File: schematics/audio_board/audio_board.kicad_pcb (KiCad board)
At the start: 2 copper layers, 69 parts, among them J1 servo ctrl, J10 charge en, J3 power, J4 pyr ctrl, J5 servo out, J6 pyr in, J7 audio ctrl, J8 speaker, J9 battery, Q1 bc847, Q2 bc847, Q3 bc847, Q7 dgm2305ux, Q8 dgm2305ux, Q9 dgm2305ux, U1 TPS613222ADBV, U2 MAX98357A, U3 TPS613222ADBV, U4 TPS613222ADBV, U8 MCP73812

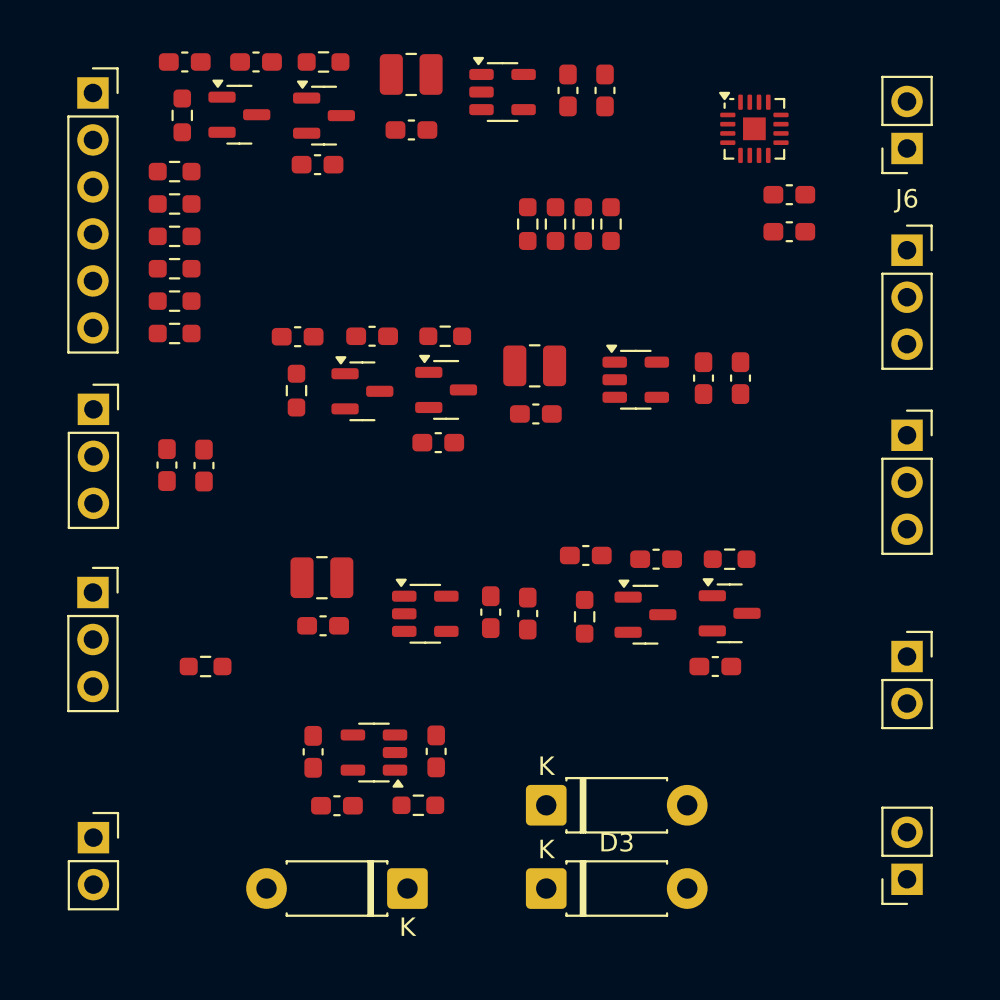
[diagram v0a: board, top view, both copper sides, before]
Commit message: a
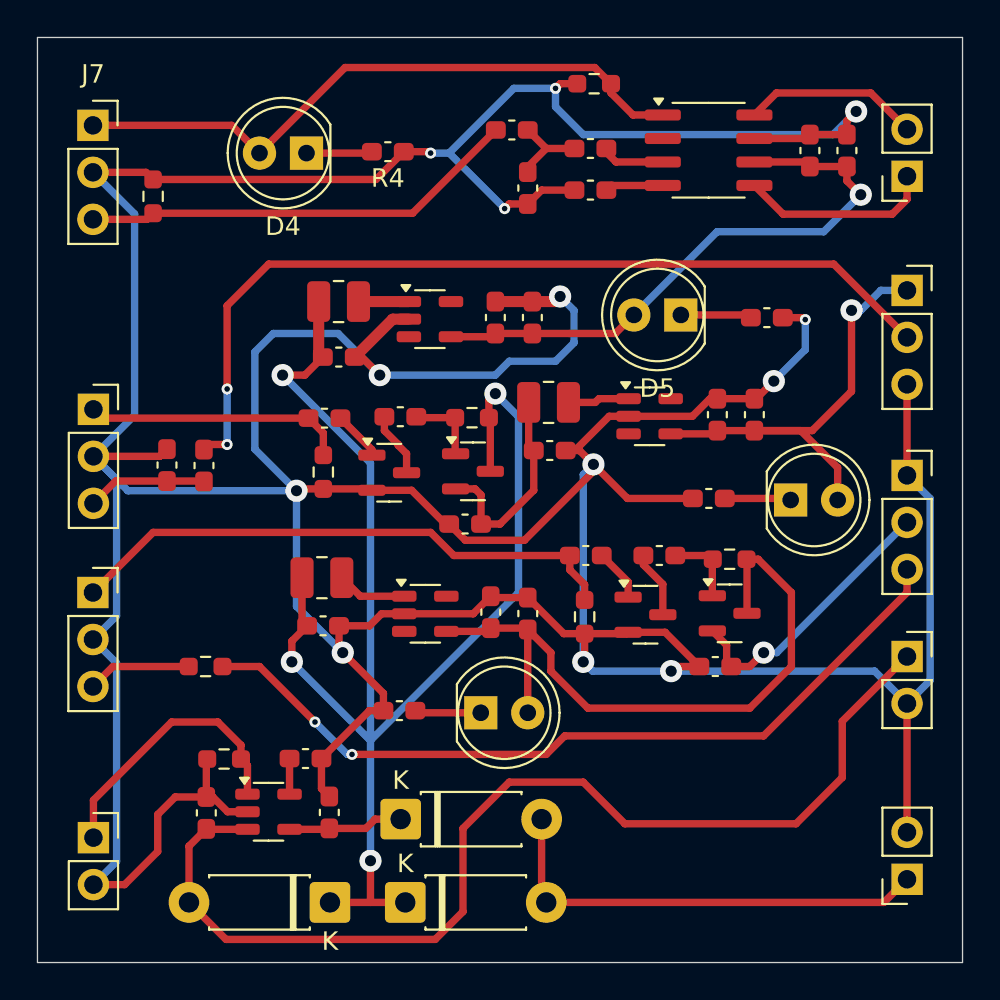
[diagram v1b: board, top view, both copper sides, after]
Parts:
- removed C16: 22u, Capacitor_SMD:C_0603_1608Metric_Pad1.08x0.95mm_HandSolder
- removed C3: 100n, Capacitor_SMD:C_0603_1608Metric_Pad1.08x0.95mm_HandSolder
- removed Q3: bc847, Package_TO_SOT_SMD:SOT-23
- removed Q9: dgm2305ux, Package_TO_SOT_SMD:SOT-23
- removed R15, R16, R18, R19, R22, R23, R24, R25: 100k, Resistor_SMD:R_0603_1608Metric_Pad0.98x0.95mm_HandSolder
- removed U2: MAX98357A, Package_DFN_QFN:TQFN-16-1EP_3x3mm_P0.5mm_EP1.23x1.23mm
- added C13: 100n, Capacitor_SMD:C_0603_1608Metric_Pad1.08x0.95mm_HandSolder, F.Cu at (79.9, 58.2)
- added C18: 100n, Capacitor_SMD:C_0603_1608Metric_Pad1.08x0.95mm_HandSolder, F.Cu at (79.9, 56.0)
- added C19: 22u, Capacitor_SMD:C_0603_1608Metric_Pad1.08x0.95mm_HandSolder, F.Cu at (93.8, 56.1)
- added C20: 100n, Capacitor_SMD:C_0603_1608Metric_Pad1.08x0.95mm_HandSolder, F.Cu at (91.8, 56.1)
- added D4: LED, LED_THT:LED_D5.0mm, F.Cu at (64.5, 56.2)
- added D5: LED, LED_THT:LED_D5.0mm, F.Cu at (84.8, 65.0)
- added D6: LED, LED_THT:LED_D5.0mm, F.Cu at (74.0, 86.5)
- added D7: LED, LED_THT:LED_D5.0mm, F.Cu at (90.7, 75.0)
- added R26: 100k, Resistor_SMD:R_0603_1608Metric_Pad0.98x0.95mm_HandSolder, F.Cu at (80.1, 52.5)
- added U5: PAM8302AAD, Package_SO:SOIC-8_3.9x4.9mm_P1.27mm, F.Cu at (86.3, 56.1)
- C2: value 22u -> 100n
- J7: footprint Connector_PinSocket_2.54mm:PinSocket_1x06_P2.54mm_Vertical -> Connector_PinSocket_2.54mm:PinSocket_1x03_P2.54mm_Vertical
- R13: value 100k -> 1k; footprint Resistor_SMD:R_0603_1608Metric_Pad0.98x0.95mm_HandSolder -> Capacitor_SMD:C_0603_1608Metric_Pad1.08x0.95mm_HandSolder
- R2, R4: value 33 -> 1k; footprint Resistor_SMD:R_0603_1608Metric_Pad0.98x0.95mm_HandSolder -> Capacitor_SMD:C_0603_1608Metric_Pad1.08x0.95mm_HandSolder
- R3: value 33 -> 100k
- moved R13 35.3 mm to (69.6, 86.4), turned to 0 degrees
- moved R12 34.4 mm to (89.4, 65.1), turned to 180 degrees
- moved R14 34.0 mm to (86.3, 74.9), turned to 0 degrees
- moved R2 18.7 mm to (75.6, 55.0)
- moved R4 15.1 mm to (68.9, 56.2), turned to 180 degrees
- moved C2 14.3 mm to (76.5, 58.1), turned to -90 degrees
- moved C6 12.9 mm to (66.3, 67.3)
- moved C1 12.9 mm to (76.8, 65.1)
- moved C17 12.9 mm to (74.8, 65.1)
- moved L1 12.9 mm to (66.3, 64.3)
- moved U1 12.9 mm to (71.2, 65.2)
- moved C8 12.9 mm to (59.1, 91.9), turned to 90 degrees
- moved R1 10.8 mm to (60.1, 89.0), turned to 180 degrees
- moved D2 9.25 mm to (69.9, 96.8)
- moved D3 8.72 mm to (69.6, 92.2)
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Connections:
- C2 pad 1: /5V_audio -> /audio_in
- C6 pad 1: /Power ctrl PYR1/pwr_out -> /Vin
- J7 pad 2: Net-(J7-Pin_2) -> GND
- J7 pad 3: Net-(J7-Pin_3) -> /audio_dac
- L1 pad 1: /Power ctrl PYR1/pwr_out -> /Vin
- R12 pad 1: /audio_en -> GND
- R13 pad 1: /Vin -> GND
- R13 pad 2: Net-(Q9-G) -> Net-(D6-K)
- R14 pad 1: Net-(Q9-G) -> GND
- R2 pad 1: Net-(J7-Pin_2) -> /audio_dac
- R2 pad 2: /lrclk -> /audio_in
- R3 pad 1: Net-(J7-Pin_3) -> GND
- R3 pad 2: /bclk -> /audio_dac
- R4 pad 1: Net-(J7-Pin_4) -> GND
- R4 pad 2: /din -> Net-(D4-K)
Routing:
- net GND: track 0.00 -> 320.8 mm, vias 0 -> 13
- net /Vin: track 0.00 -> 78.2 mm, vias 0 -> 4
- net /Vbatt: track 0.00 -> 58.9 mm
- net /pyr_in: track 0.00 -> 48.2 mm, vias 0 -> 2
- net Net-(J5-Pin_3): track 0.00 -> 43.8 mm, vias 0 -> 2
- net /5V_servo: track 0.00 -> 36.6 mm
- net /audio_en: track 0.00 -> 34.7 mm
- net /5V_audio: track 0.00 -> 32.7 mm, vias 0 -> 1
- net /Power ctrl/en: track 0.00 -> 30.4 mm
- net /5V_pyr: track 0.00 -> 25.6 mm, vias 0 -> 1
- net /pwr+: track 0.00 -> 24.6 mm
- net /audio_dac: track 0.00 -> 23.8 mm
- net /Power ctrl/pwr_out: track 0.00 -> 15.1 mm, vias 0 -> 1
- net /charge_en: track 0.00 -> 15.1 mm
- net /pyr_en: track 0.00 -> 14.2 mm
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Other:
- board outline added: 50 x 50 mm
